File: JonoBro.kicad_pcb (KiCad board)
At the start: 2 copper layers, 43.5 x 34 mm, 9 parts, among them J1 Conn_01x02_Pin, J2 Conn_01x02_Pin, J3 Conn_01x02_Pin, J4 Conn_01x02_Pin, Q1 PSMN5R2-60YL, U1 ATtiny25V-10M, U2 HT75xx-1-SOT89

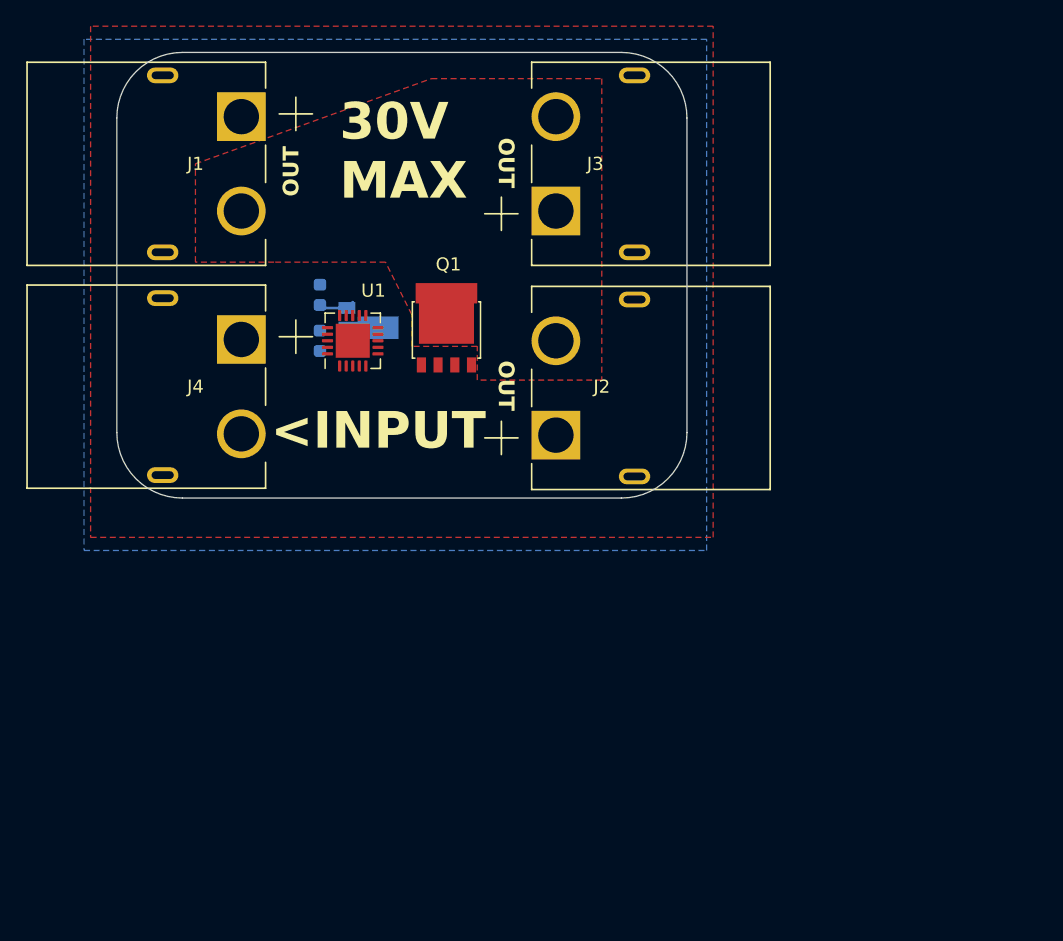
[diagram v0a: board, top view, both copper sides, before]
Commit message: seems good to me
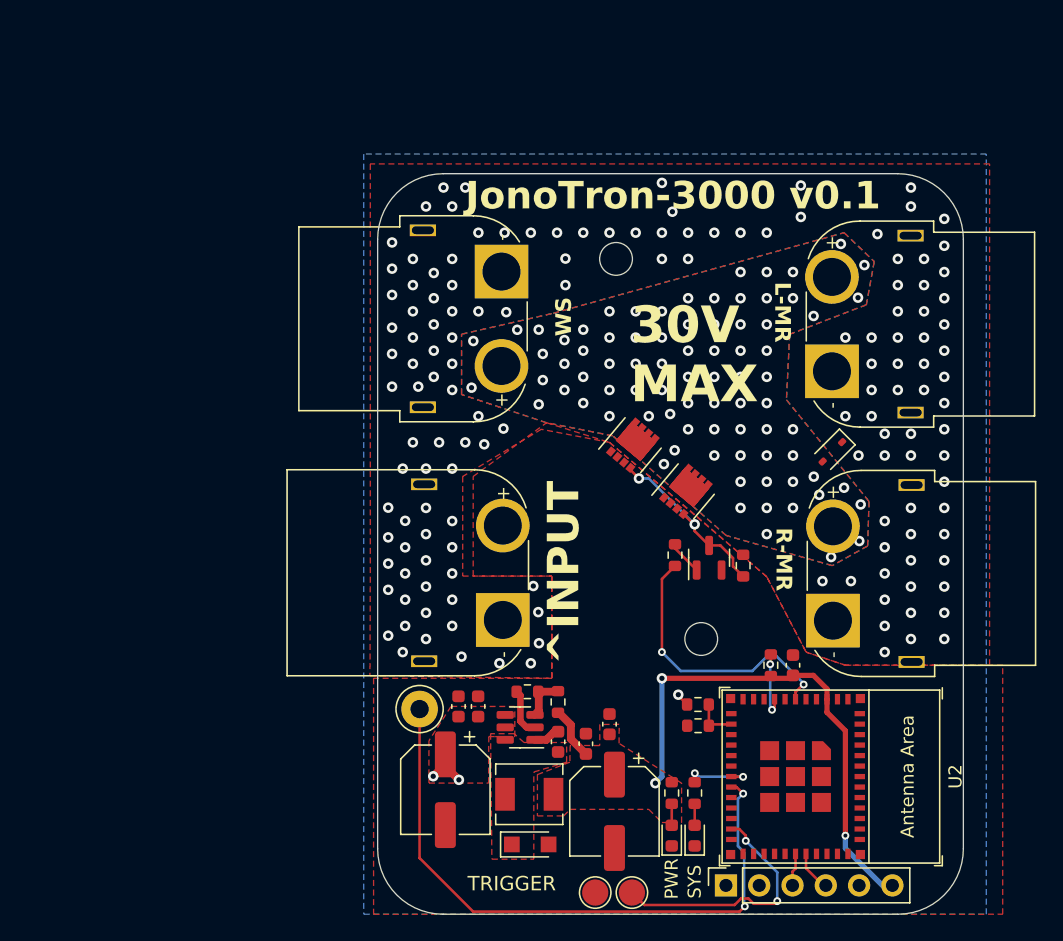
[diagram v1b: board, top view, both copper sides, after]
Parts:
- added C3: 100nF, Capacitor_SMD:C_0603_1608Metric, F.Cu at (126.1, 104.4)
- added C4: 100nF, Capacitor_SMD:C_0603_1608Metric, F.Cu at (132.2, 107.1)
- added C5: 22uF, Capacitor_SMD:CP_Elec_6.3x5.4, F.Cu at (136.5, 112.4)
- added C6: 10uF, Capacitor_SMD:C_0603_1608Metric, F.Cu at (136.1, 105.8)
- added C7: 100nF, Capacitor_SMD:C_0603_1608Metric, F.Cu at (134.3, 107.2)
- added C8: 100nF, Capacitor_SMD:C_0603_1608Metric, F.Cu at (150.1, 101.3)
- added D1: PMEG6020ER, Diode_SMD:Nexperia_CFP3_SOD-123W, F.Cu at (130.0, 114.9)
- added D2: LED_Small, LED_SMD:LED_0603_1608Metric, F.Cu at (140.8, 114.3)
- added D3: LED_Small, LED_SMD:LED_0603_1608Metric, F.Cu at (142.6, 114.3)
- added D4: 1N5819WS, Diode_SMD:D_SOD-323, F.Cu at (153.1, 85.0)
- added H1: MountingHole, MountingHole:MountingHole_2.5mm, F.Cu at (143.1, 99.3)
- added H2: MountingHole, MountingHole:MountingHole_2.5mm, F.Cu at (136.6, 70.3)
- added J5: Conn_01x06_Socket, Connector_PinSocket_2.54mm:PinSocket_1x06_P2.54mm_Vertical, F.Cu at (145.0, 118.1)
- added L1: 10uH, Inductor_SMD:L_Chilisin_BMRA00040415, F.Cu at (130.0, 111.1)
- added Q2: MMBT3904, Package_TO_SOT_SMD:SOT-23, F.Cu at (143.7, 93.1)
- added Q3: CSD19537Q3, Package_SON:VSON-8_3.3x3.3mm_P0.65mm_NexFET, F.Cu at (141.9, 88.0)
- added R1: 13k, Resistor_SMD:R_0603_1608Metric, F.Cu at (132.2, 104.1)
- added R2: 4.3k, Resistor_SMD:R_0603_1608Metric, F.Cu at (129.8, 103.3)
- added R3: 2.2k, Resistor_SMD:R_0603_1608Metric, F.Cu at (140.8, 111.0)
- added R4: 2.2k, Resistor_SMD:R_0603_1608Metric, F.Cu at (142.8, 105.9)
- added R5: 13k, Resistor_SMD:R_0603_1608Metric, F.Cu at (148.4, 101.3)
- added R6: 2.2k, Resistor_SMD:R_0603_1608Metric, F.Cu at (142.6, 111.0)
- added R7: 13k, Resistor_SMD:R_0603_1608Metric, F.Cu at (142.8, 104.3)
- added R8: 1k, Resistor_SMD:R_0603_1608Metric, F.Cu at (141.1, 92.9)
- added R9: 13k, Resistor_SMD:R_0603_1608Metric, F.Cu at (146.3, 93.7)
- added TP1: TestPoint, TestPoint:TestPoint_Pad_D2.0mm, F.Cu at (137.8, 118.6)
- added TP2: TestPoint, TestPoint:TestPoint_Pad_D2.0mm, F.Cu at (135.0, 118.6)
- added TP3: TestPoint, TestPoint:TestPoint_Loop_D3.50mm_Drill1.4mm_Beaded, F.Cu at (121.6, 104.6)
- C1: value 10uF -> 220uF; footprint Capacitor_SMD:C_0603_1608Metric -> Capacitor_SMD:CP_Elec_6.3x7.7; moved to F.Cu
- C2: moved to F.Cu
- J1, J2, J3: footprint XT60PW-M:AMASS_XT60PW-M -> Acea:AMASS_XT60PW-F_1x02_P7.20mm_Horizontal
- J4: footprint XT60PW-M:AMASS_XT60PW-M -> Acea:AMASS_XT60PW-M_1x02_P7.20mm_Horizontal
- Q1: value PSMN5R2-60YL -> CSD19537Q3; footprint Package_TO_SOT_SMD:LFPAK56 -> Package_SON:VSON-8_3.3x3.3mm_P0.65mm_NexFET
- U1: value ATtiny25V-10M -> AOZ1280CI; footprint Package_DFN_QFN:QFN-20-1EP_4x4mm_P0.5mm_EP2.6x2.6mm -> Package_TO_SOT_SMD:SOT-23-6
- U2: value HT75xx-1-SOT89 -> ESP32-C3-MINI-1; footprint Package_TO_SOT_SMD:SOT-89-3 -> Espressif:ESP32-C3-MINI-1; moved to F.Cu
- moved U2 49.0 mm to (153.0, 109.7), turned to -90 degrees
- moved C1 35.6 mm to (123.6, 110.8)
- moved C2 33.1 mm to (124.6, 104.4)
- moved U1 32.1 mm to (129.3, 106.0), turned to 180 degrees
- moved J4 31.5 mm to (128.0, 97.8)
- moved J1 27.1 mm to (127.8, 71.2)
- moved J2 23.3 mm to (153.1, 97.9)
- moved J3 21.9 mm to (153.1, 78.8)
- moved Q1 16.7 mm to (137.9, 84.5), turned to 50 degrees
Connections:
- C2 pad 1: +3.3V -> +12V
- Q1 pad 4: unconnected-(Q1-G-Pad4) -> Net-(Q1-G)
- U1 pad 1: unconnected-(U1-~{RESET}/PB5-Pad1) -> Net-(U1-BST)
- U1 pad 2: unconnected-(U1-XTAL1/PB3-Pad2) -> GND
- U1 pad 3: unconnected-(U1-NC-Pad3) -> Net-(U1-FB)
- U1 pad 4: unconnected-(U1-NC-Pad4) -> +12V
- U1 pad 5: unconnected-(U1-XTAL2/PB4-Pad5) -> +12V
- U1 pad 6: unconnected-(U1-NC-Pad6) -> Net-(D1-K)
- U2 pad 2: +12V -> GND
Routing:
- net SWITCH: track 0.00 -> 48.1 mm, vias 0 -> 2
- net +3.3V: track 2.78 -> 43.1 mm, vias 0 -> 3
- net MOSFET: track 0.00 -> 21.7 mm, vias 0 -> 2
- net Net-(U2-GPIO9): track 0.00 -> 19.2 mm, vias 0 -> 2
- net Net-(Q1-G): track 0.00 -> 14.2 mm, vias 0 -> 2
- net +12V: track 0.00 -> 5.49 mm, vias 0 -> 146
- net SYS_LED: track 0.00 -> 5.46 mm, vias 0 -> 2
- net Net-(U2-EN/CHIP_PU): track 0.00 -> 5.19 mm, vias 0 -> 2
- net GND: track 0.00 -> 3.60 mm
- net VIn: track 0.00 -> 3.38 mm
- net Net-(U1-FB): track 0.00 -> 3.37 mm
- net Net-(J5-Pin_4): track 0.00 -> 3.23 mm
- net Net-(J5-Pin_3): track 0.00 -> 2.71 mm
- net Net-(Q2-B): track 0.00 -> 2.65 mm
- net Net-(U1-BST): track 0.00 -> 2.02 mm
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- added copper zone on F.Cu, net +12V
- added copper zone on F.Cu, net +3.3V
- added copper zone on F.Cu, net Net-(D1-K)
- added copper zone on B.Cu, net Net-(D4-A)
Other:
- board size 43.5 x 34 mm -> 44.7 x 56.5 mm
- board text added: "JonoTron-3000 v0.1"
- board text added: "L-MR"
- board text added: "PWR"
- board text added: "R-MR"
- board text added: "SYS"
- board text added: "TRIGGER"
- board text added: "WS"
- board text added: "^INPUT"
- board text removed: "<INPUT"
- board text removed: "OUT"
